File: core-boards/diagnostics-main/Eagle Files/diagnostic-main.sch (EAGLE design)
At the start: 37 parts, among them J1 A118090TR-ND, J2 3M15451-ND, J4 B2PS-VH(LF)(SN), Q1 16 MHz, U1 ATMEGA2560-16AU, U2 296-38653-1-ND, U3 MCP2551T-I/SN, U6 TXB0106PWR, U7 LM1085ISX-5.0/NOPB, U8 LP2985IM5X-3.3/NOPB, X1 22-23-2031, X2 B6B-EH-A(LF)(SN), X3 CC1101, X5 22-23-2031, X8 WM4803-ND

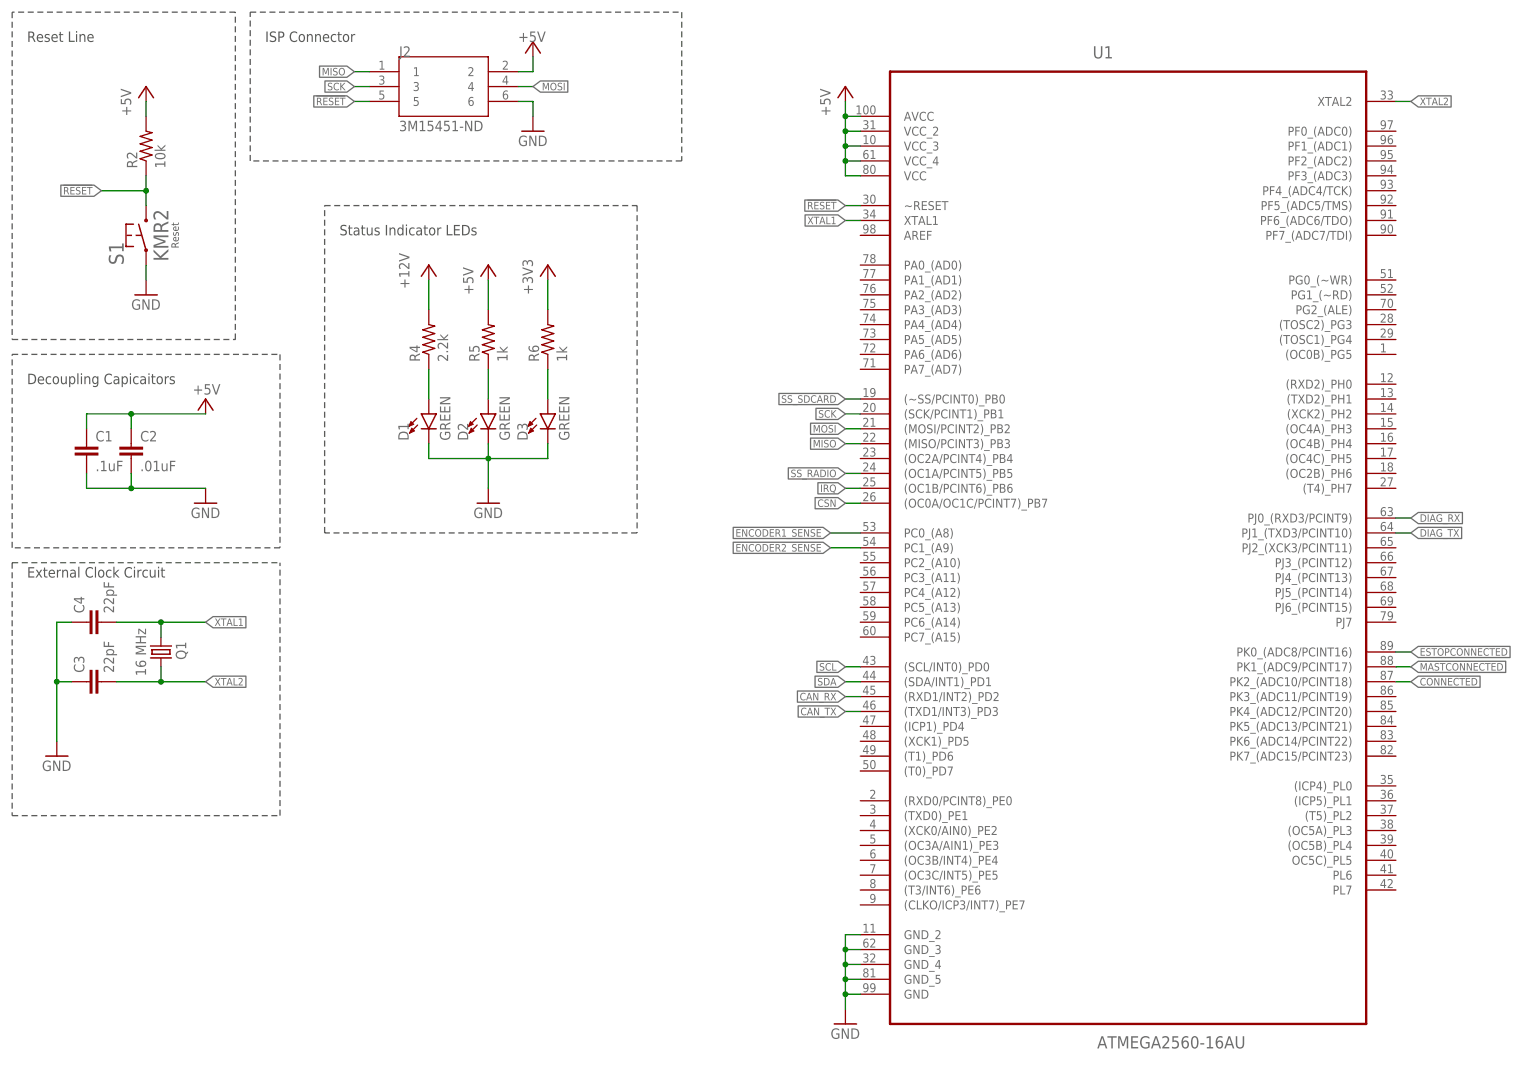
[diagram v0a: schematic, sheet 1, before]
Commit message: Design Review Changes
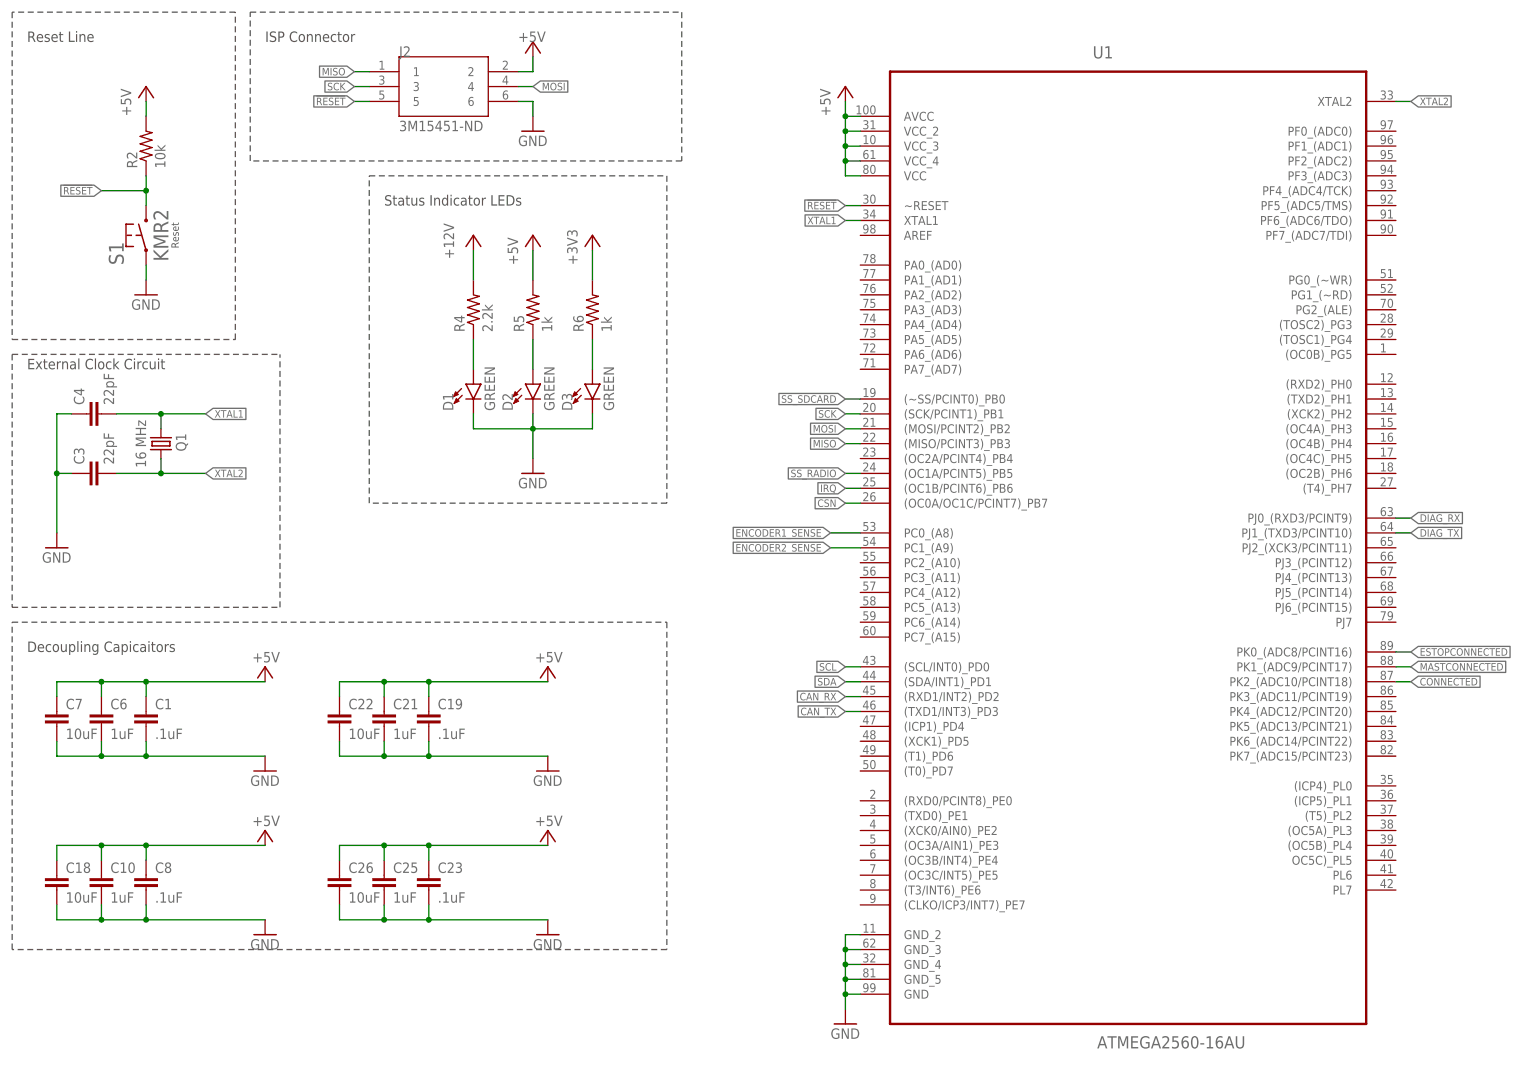
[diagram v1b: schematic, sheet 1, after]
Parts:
- added C10, C21, C25, C6: 1uF, rcl:C-EUC0402
- added C18, C22, C26, C7: 10uF, rcl:C-EUC0805
- added C19, C23, C8, C9: .1uF, rcl:C-EUC0603
- C2: value .01uF -> .1uF
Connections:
- net +3V3: now also C2.1
- net +5V: now also C10.1, C18.1, C19.1, C21.1, C22.1, C23.1, C25.1, C26.1, C6.1, C7.1, C8.1, C9.1; no longer C2.1
- net GND: now also C10.2, C18.2, C19.2, C21.2, C22.2, C23.2, C25.2, C26.2, C6.2, C7.2, C8.2, C9.2
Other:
- moved on the sheet: C1, C3, C4, D1, D2, D3, Q1, R1, R3, R4, R5, R6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
